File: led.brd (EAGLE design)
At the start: 100 x 80 mm, 22 parts, among them U1 TPS92513HV

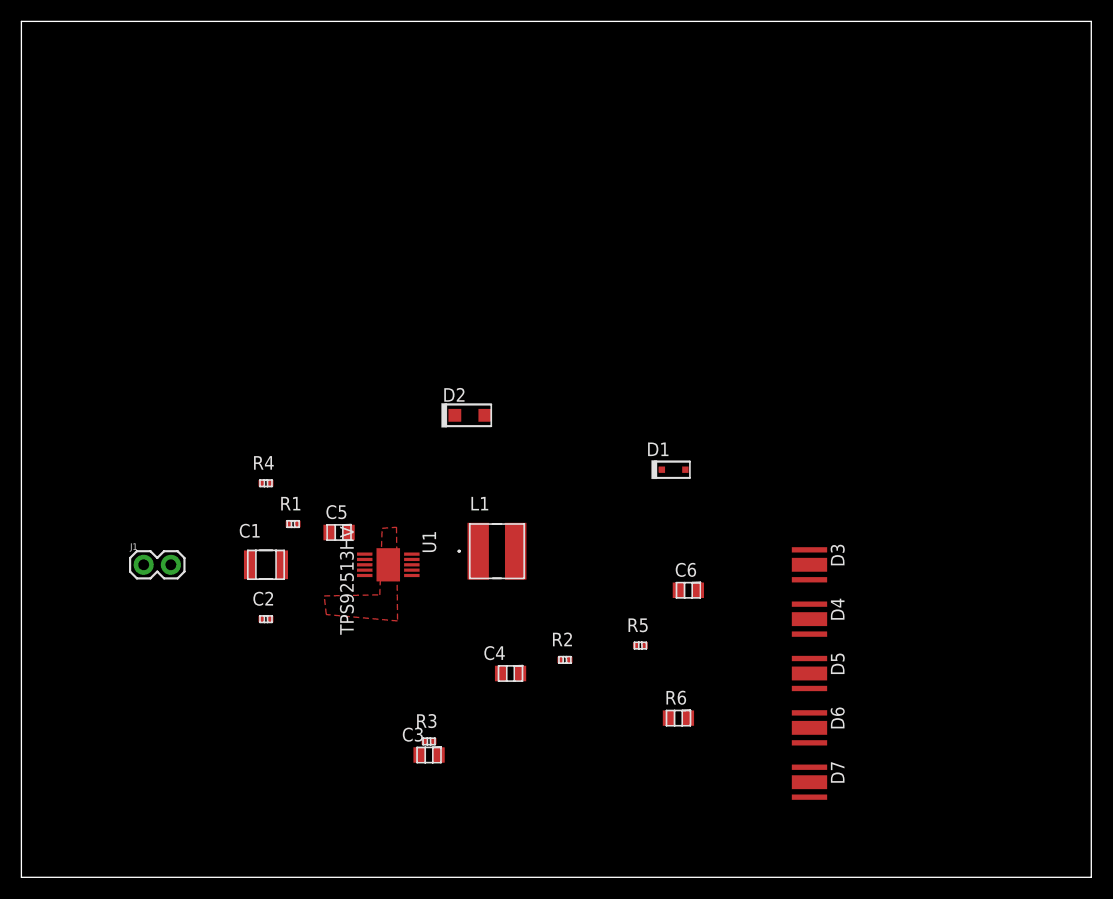
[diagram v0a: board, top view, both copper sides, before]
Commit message: save
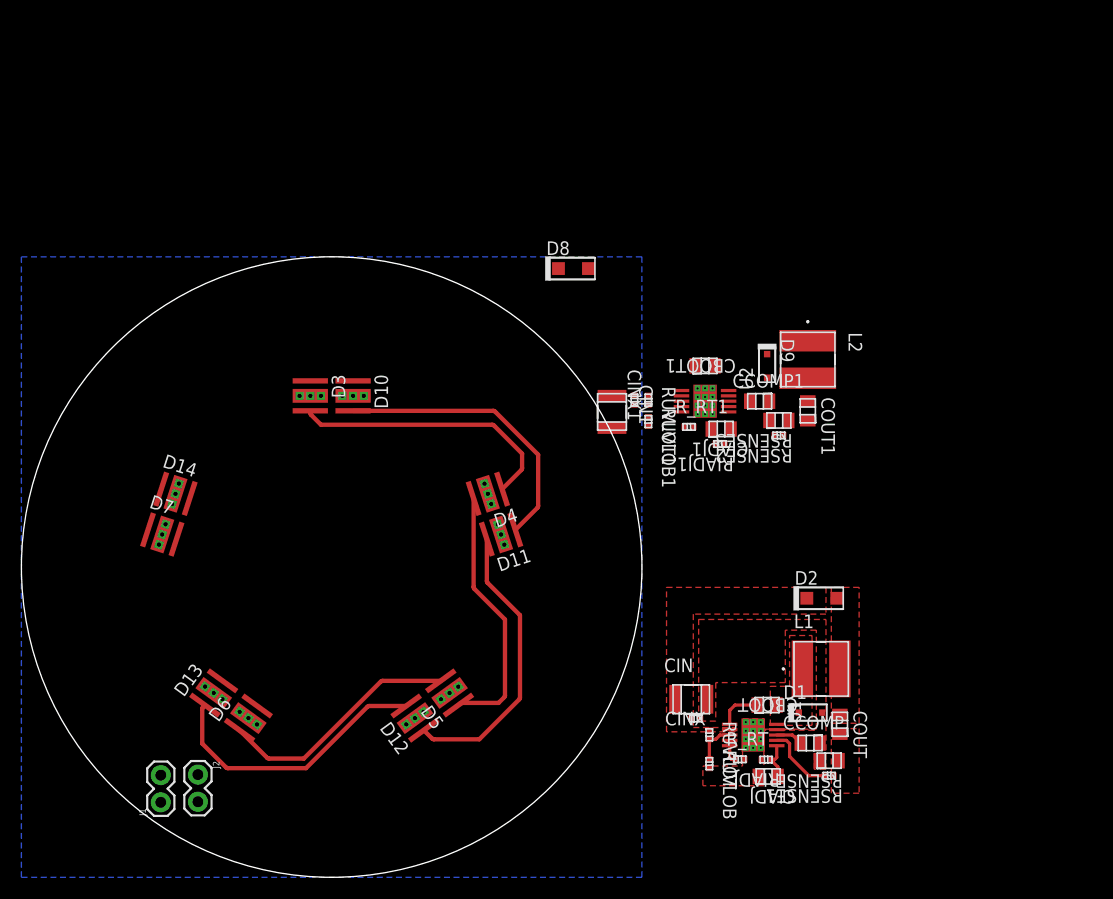
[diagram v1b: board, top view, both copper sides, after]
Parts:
- removed C1: GRM32ER71J106KA12L, derek:1210_280
- removed C2: GCM155R71H103KA55D, derek:0402
- removed C3: CC0805KRX7R9BB103, derek:CC0805KRX7R9BB103
- removed C4: CC0805KRX7R8BB104, derek:CC0805KRX7R8BB104
- removed C5: 08053C104KAT2A, derek:0805
- removed C6: GMK212B7105KG-T, derek:GMK212B7105KG-T
- removed R1: CRCW0402121KFKED, derek:CRCW0402121KFKED
- removed R2: CRCW04027K68FKED, derek:CRCW04027K68FKED
- removed R3, R5: CRCW04021K00FKED, derek:CRCW04021K00FKED
- removed R4: CRCW0402162KFKED, derek:CRCW0402162KFKED
- removed R6: CRM0805-FX-R510ELF, derek:CRM0805-FX-R510ELF
- added CBOOT, CBOOT1: 08053C104KAT2A, derek:0805
- added CCOMP, CCOMP1: CC0805KRX7R8BB104, derek:CC0805KRX7R8BB104
- added CIADJ, CIADJ1: CC0805KRX7R9BB103, derek:CC0805KRX7R9BB103
- added CIN, CIN1: GRM32ER71J106KA12L, derek:1210_280
- added CINX, CINX1: GCM155R71H103KA55D, derek:0402
- added COUT, COUT1: GMK212B7105KG-T, derek:GMK212B7105KG-T
- added D10, D11, D12, D13, D14: XPGWHT, derek:XLAMP-XPG
- added D8: PMEG6010CEH,115, derek:SOD-123F
- added D9: BAT54WSTR, derek:SOD-323
- added J2: (no value), derek:1X02
- added L2: 74408943220, derek:IND_WE-SPC
- added RIADJ, RIADJ1, RSENSE1, RSENSE2: CRCW04021K00FKED, derek:CRCW04021K00FKED
- added RSENSE, RSENSE3: CRM0805-FX-R510ELF, derek:CRM0805-FX-R510ELF
- added RUVLOB, RUVLOB1: CRCW04027K68FKED, derek:CRCW04027K68FKED
- added RUVLOT, RUVLOT1: CRCW0402121KFKED, derek:CRCW0402121KFKED
- added R_RT, R_RT1: CRCW0402162KFKED, derek:CRCW0402162KFKED
- added U2: TPS92513HV, derek:TPS92513
- moved D7 64.8 mm to (13.2, 32.0), turned to 342 degrees
- moved D6 52.5 mm to (21.2, 14.9), turned to 54 degrees
- moved D3 49.3 mm to (27.0, 45.0)
- moved U1 37.6 mm to (68.4, 13.3)
- moved D2 37.1 mm to (74.8, 26.1)
- moved D5 33.7 mm to (40.0, 17.2), turned to 126 degrees
- moved D4 32.3 mm to (43.6, 35.8), turned to 198 degrees
- moved L1 32.2 mm to (74.8, 19.5)
- moved D1 26.1 mm to (73.8, 15.4)
- moved J1 22.3 mm to (13.0, 7.01), turned to 90 degrees
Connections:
- removed net GND: C1.2, C2.2, C3.2, C4.2, D1.2, J1.1, R2.2, R3.2, R4.2, R6.2, U1.9, U1.GND
- new net 24V: CIN.1, CIN1.1, CINX.1, CINX1.1, D2.1, D8.1, J1.2, RUVLOT.1, RUVLOT1.1, U1.2, U2.2
- new net GND-ISO: CCOMP.2, CCOMP1.2, CIADJ.2, CIADJ1.2, CIN.2, CIN1.2, CINX.2, CINX1.2, D1.2, D10.GND, D10.P$1, D10.P$2, D10.P$3, D11.GND, D11.P$1, D11.P$2, D11.P$3, D12.GND, D12.P$1, D12.P$2, D12.P$3, D13.GND, D13.P$1, D13.P$2, D13.P$3, D14.GND, D14.P$1, D14.P$2, D14.P$3, D3.GND, D3.P$1, D3.P$2, D3.P$3, D4.GND, D4.P$1, D4.P$2, D4.P$3, D5.GND, D5.P$1, D5.P$2, D5.P$3, D6.GND, D6.P$1, D6.P$2, D6.P$3, D7.GND, D7.P$1, D7.P$2, D7.P$3, D9.2, J1.1, RIADJ.2, RIADJ1.2, RSENSE.2, RSENSE3.2, RUVLOB.2, RUVLOB1.2, R_RT.2, R_RT1.2, U1.9, U1.GND-ISO, U1.P$1, U1.P$10, U1.P$11, U1.P$12, U1.P$2, U1.P$3, U1.P$4, U1.P$5, U1.P$6, U1.P$7, U1.P$8, U1.P$9, U2.9, U2.GND-ISO, U2.P$1, U2.P$10, U2.P$11, U2.P$12, U2.P$2, U2.P$3, U2.P$4, U2.P$5, U2.P$6, U2.P$7, U2.P$8, U2.P$9
- new net N$1: RUVLOB1.1, RUVLOT1.2, U2.3
- new net N$16: CBOOT1.1, D9.1, L2.1, U2.10
- new net N$17: COUT1.2, D14.C, RSENSE2.1, RSENSE3.1
- new net N$18: COUT1.1, D10.A, D8.2, L2.2
- new net N$19: R_RT1.1, U2.5
- new net N$20: CCOMP1.1, U2.8
- new net N$21: CBOOT1.2, U2.1
- new net N$22: RSENSE2.2, U2.7
- new net N$23: D10.C, D11.A
- new net N$24: D11.C, D12.A
- new net N$25: D12.C, D13.A
- new net N$26: D13.C, D14.A
- new net PDIM1: J2.1, U1.4
- new net PDIM2: J2.2, U2.4
- net N$10: now also CBOOT.2; no longer C5.2
- net N$11: now also RSENSE1.2; no longer R5.2
- net N$2: now also CIADJ.1, RIADJ.1; no longer C3.1, R3.1
- net N$3: now also RUVLOB.1, RUVLOT.2; no longer R1.2, R2.1
- net N$4: now also CIADJ1.1, RIADJ1.1, U2.6; no longer C1.1, C2.1, D2.1, J1.2, R1.1, U1.2
- net N$5: now also CBOOT.1; no longer C5.1
- net N$6: now also COUT.2, RSENSE.1, RSENSE1.1; no longer C6.2, R5.1, R6.1
- net N$7: now also COUT.1; no longer C6.1
- net N$8: now also R_RT.1; no longer R4.1
- net N$9: now also CCOMP.1; no longer C4.1
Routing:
- net N$24: track 0.00 -> 27.1 mm
- net N$23: track 0.00 -> 26.9 mm
- net N$25: track 0.00 -> 26.1 mm
- net N$12: track 0.00 -> 25.7 mm
- net N$13: track 0.00 -> 24.4 mm
- net N$14: track 0.00 -> 22.9 mm
- net N$11: track 0.00 -> 6.55 mm
- net N$10: track 0.00 -> 4.11 mm
- net N$3: track 0.00 -> 3.93 mm
- net N$2: track 0.00 -> 3.62 mm
- net N$9: track 0.00 -> 2.53 mm
- net N$8: track 0.00 -> 1.71 mm
- added copper zone on layer 1, net 24V
- added copper zone on layer 1, net GND-ISO
- added copper zone on layer 16, net GND-ISO
- added copper zone on layer 1, net N$5
- added copper zone on layer 1, net N$6
- added copper zone on layer 1, net N$7
- removed copper zone on layer 1, net GND
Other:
- board size 100 x 80 mm -> 58 x 58 mm
